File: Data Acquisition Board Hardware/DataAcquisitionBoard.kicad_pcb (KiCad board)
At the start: 2 copper layers, 99.1 x 68.6 mm, 14 parts, among them P1 BNC, P2 BNC, P3 BNC, P4 BNC, P5 CONN_01X04

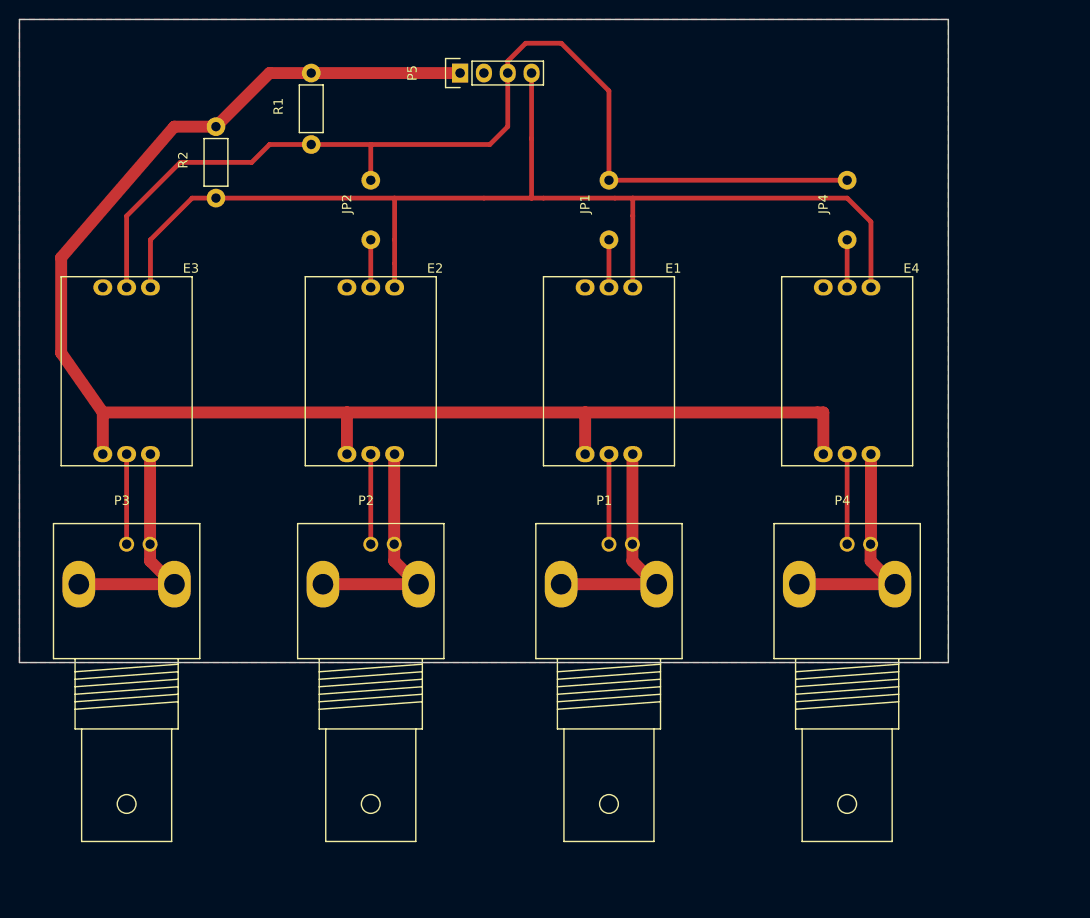
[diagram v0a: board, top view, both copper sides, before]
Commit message: Finalized PCB layout
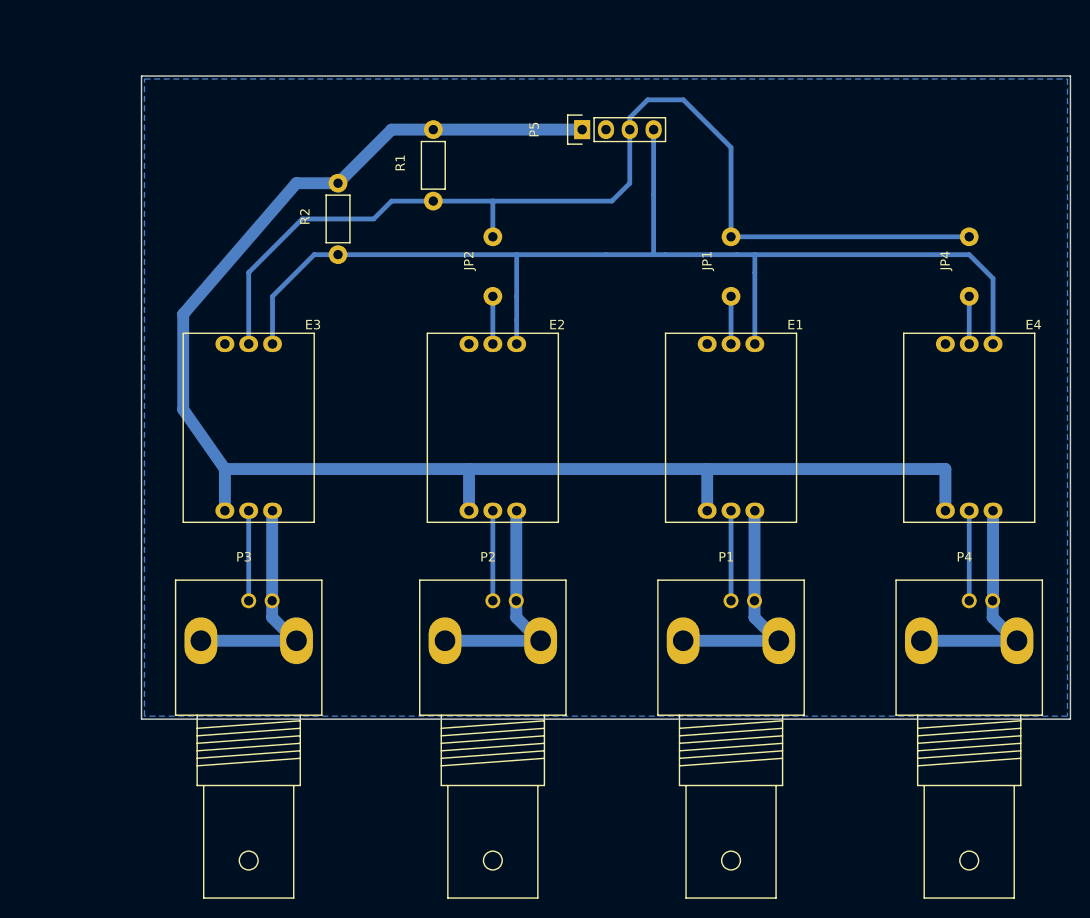
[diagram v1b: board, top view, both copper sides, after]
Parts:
- moved E4 14.3 mm to (154.6, 127.3)
- moved JP4 14.3 mm to (154.6, 113.3)
- moved P4 14.3 mm to (154.6, 150.8)
- moved E1 14.3 mm to (129.2, 127.3)
- moved E2 14.3 mm to (103.8, 127.3)
- moved E3 14.3 mm to (77.8, 127.3)
- moved JP1 14.3 mm to (129.2, 113.3)
- moved JP2 14.3 mm to (103.8, 113.3)
- moved P1 14.3 mm to (129.2, 150.8)
- moved P2 14.3 mm to (103.8, 150.8)
- moved P3 14.3 mm to (77.8, 150.8)
- moved P5 14.3 mm to (113.3, 95.6)
- moved R1 14.3 mm to (97.5, 103.2)
- moved R2 14.3 mm to (87.3, 108.9)
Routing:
- added copper zone on B.Cu, net GND
- removed copper zone on F.Cu, net GND
